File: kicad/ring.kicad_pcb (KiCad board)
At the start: 2 copper layers, 44.5 x 50 mm, 4 parts, among them J1 Conn_01x02, U1 ESP32-WROOM-E

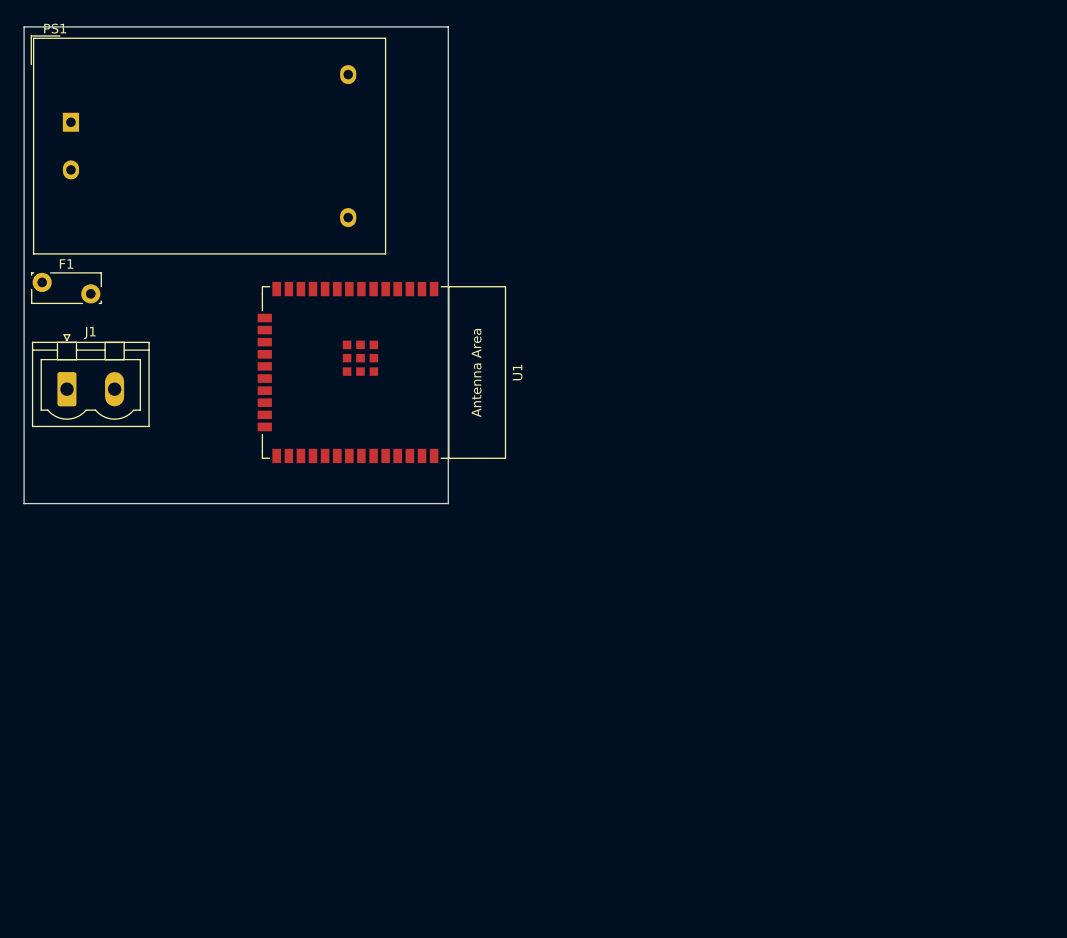
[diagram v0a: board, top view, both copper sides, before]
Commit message: init
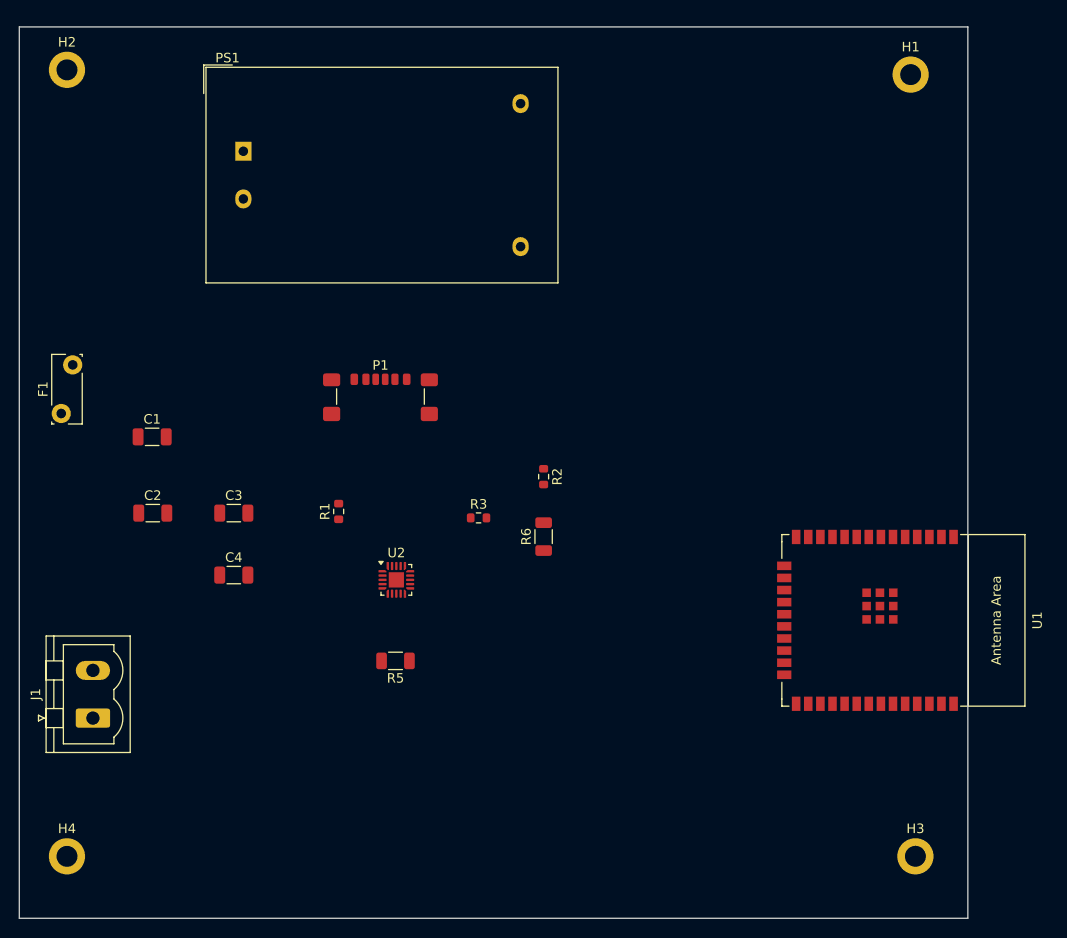
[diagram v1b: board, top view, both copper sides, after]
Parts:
- added C1: 1µF, Capacitor_SMD:C_1206_3216Metric, F.Cu at (113.9, 93.0)
- added C2: 100nF, Capacitor_SMD:C_1206_3216Metric, F.Cu at (114.0, 101.0)
- added C3: 4,7µF, Capacitor_SMD:C_1206_3216Metric, F.Cu at (122.5, 101.0)
- added C4: 0,1µF, Capacitor_SMD:C_1206_3216Metric, F.Cu at (122.5, 107.5)
- added H1: MountingHole, MountingHole:MountingHole_2.2mm_M2_DIN965_Pad, F.Cu at (193.5, 55.0)
- added H2: MountingHole, MountingHole:MountingHole_2.2mm_M2_DIN965_Pad, F.Cu at (105.0, 54.5)
- added H3: MountingHole, MountingHole:MountingHole_2.2mm_M2_DIN965_Pad, F.Cu at (194.0, 137.0)
- added H4: MountingHole, MountingHole:MountingHole_2.2mm_M2_DIN965_Pad, F.Cu at (105.0, 137.0)
- added P1: USB_C_Plug_USB2.0, Connector_USB:USB_C_Receptacle_GCT_USB4135-GF-A_6P_TopMnt_Horizontal, F.Cu at (137.9, 90.0)
- added R1: 5.1K, Resistor_SMD:R_0603_1608Metric, F.Cu at (133.5, 100.8)
- added R2: 22K, Resistor_SMD:R_0603_1608Metric, F.Cu at (155.0, 97.2)
- added R3: 47K5, Resistor_SMD:R_0603_1608Metric, F.Cu at (148.2, 101.5)
- added R5: 2K, Resistor_SMD:R_1206_3216Metric, F.Cu at (139.5, 116.5)
- added R6: 10K, Resistor_SMD:R_1206_3216Metric, F.Cu at (155.0, 103.5)
- added U2: CP2102N-Axx-xQFN20, Package_DFN_QFN:QFN-20-1EP_3x3mm_P0.45mm_EP1.6x1.6mm, F.Cu at (139.6, 108.0)
- moved U1 60.4 mm to (191.0, 112.2)
- moved J1 34.6 mm to (107.7, 122.5), turned to 90 degrees
- moved PS1 18.3 mm to (123.5, 63.0)
- moved F1 13.9 mm to (104.4, 90.5), turned to 90 degrees
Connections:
- PS1 pad 3: GND -> unconnected-(PS1--Vout-Pad3)
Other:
- board size 44.5 x 50 mm -> 99.5 x 93.5 mm
